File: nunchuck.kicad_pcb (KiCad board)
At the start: 2 copper layers, 117.9 x 118.2 mm, 56 parts, among them J2 USB_C_Receptacle_USB2.0_14P, J3 USB_C_Receptacle_USB2.0_14P, SW1 BOOT, SW2 RESET, SW3 BOOT, SW4 RESET, U1 CH552T, U2 CH552T, U3 USBLC6-2SC6, U4 USBLC6-2SC6

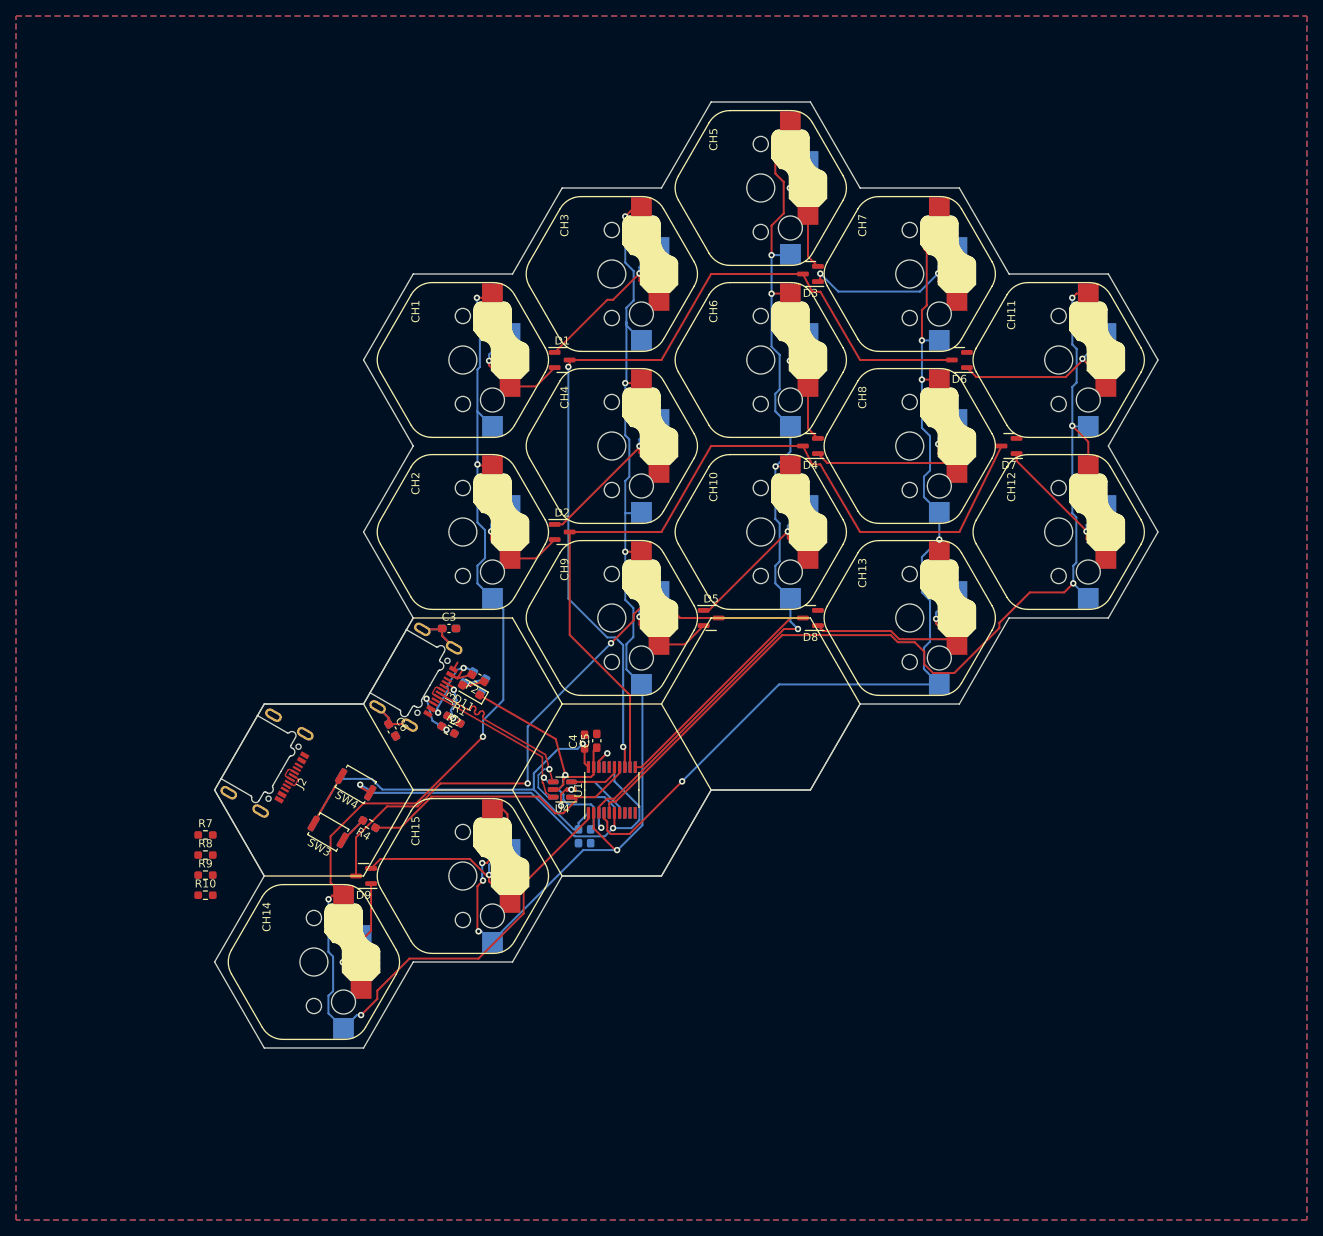
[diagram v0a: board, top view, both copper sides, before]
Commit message: before hexing
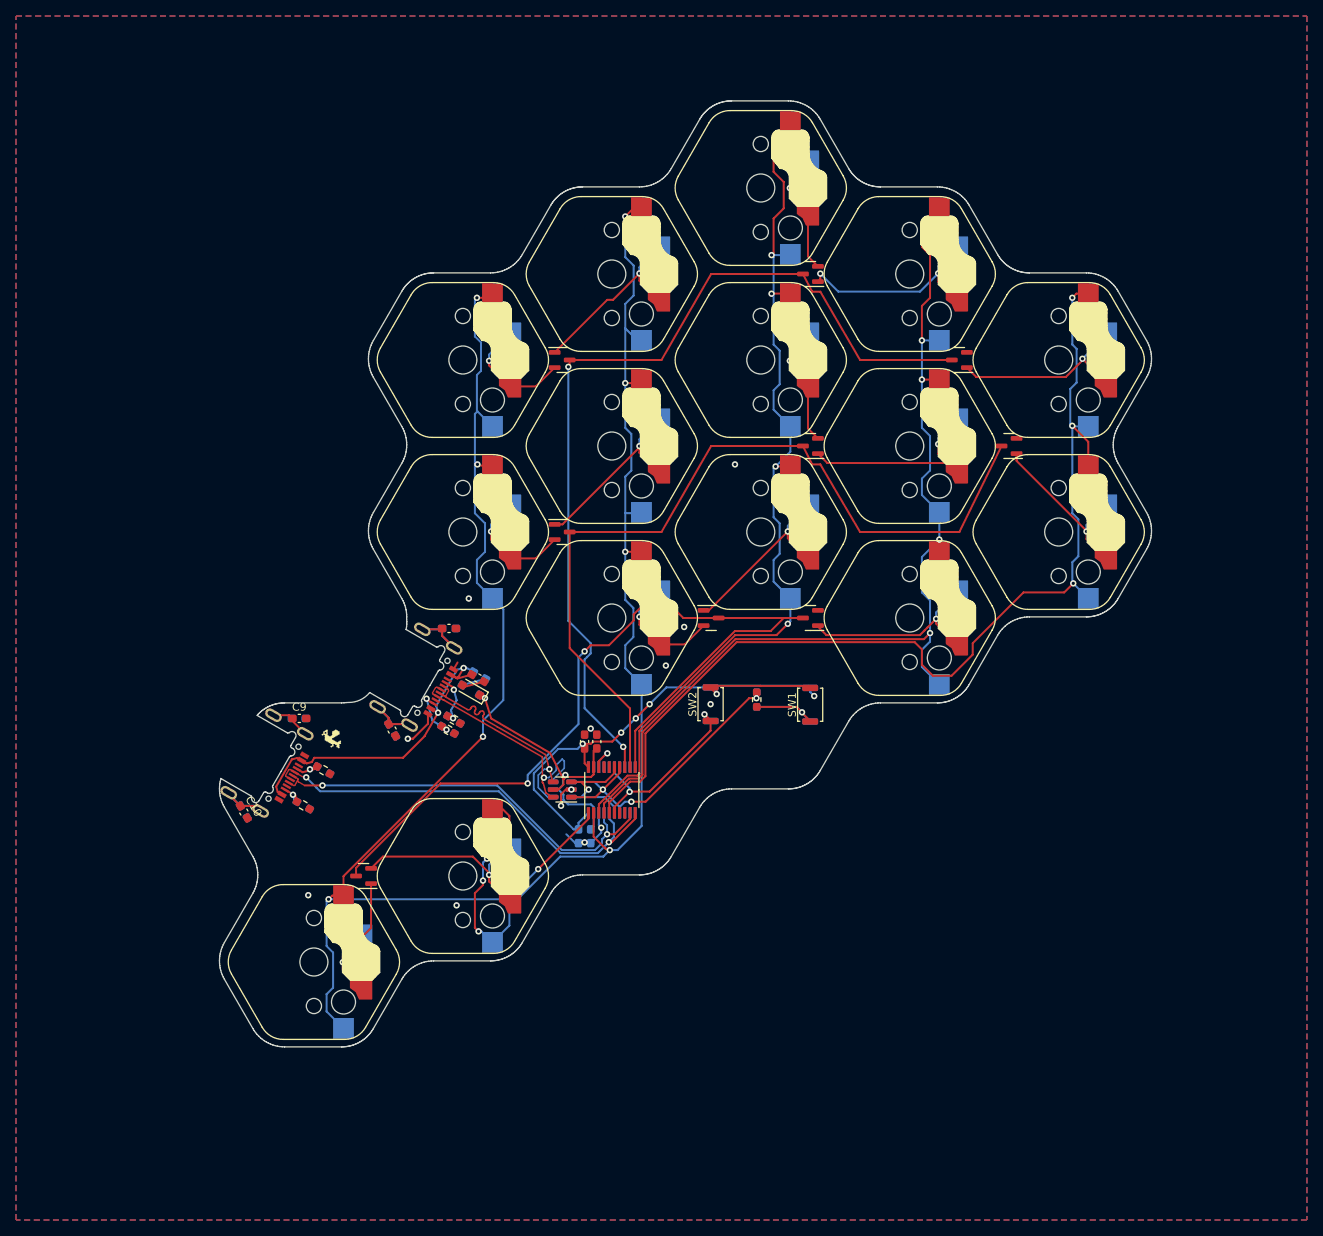
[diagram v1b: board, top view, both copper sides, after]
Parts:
- added C10: 1uF, Capacitor_SMD:C_0603_1608Metric_Pad1.08x0.95mm_HandSolder, F.Cu at (59.5, 110.3)
- added C11: 1uF, Capacitor_SMD:C_0603_1608Metric_Pad1.08x0.95mm_HandSolder, B.Cu at (59.5, 110.2)
- added C12: 1uF, Capacitor_SMD:C_0603_1608Metric_Pad1.08x0.95mm_HandSolder, B.Cu at (66.4, 98.6)
- added C9: 1uF, Capacitor_SMD:C_0603_1608Metric_Pad1.08x0.95mm_HandSolder, F.Cu at (66.4, 98.6)
- R10, R9, SW3, SW4: moved to B.Cu
- SW1, SW2: moved to F.Cu
- moved SW1 62.3 mm to (130.3, 96.8), turned to 90 degrees
- moved SW3 62.3 mm to (130.3, 96.8), turned to 90 degrees
- moved R3 50.9 mm to (123.6, 96.2), turned to -90 degrees
- moved R4 50.9 mm to (123.6, 96.2), turned to -90 degrees
- moved SW2 45.5 mm to (117.9, 96.8), turned to 90 degrees
- moved SW4 45.5 mm to (117.9, 96.8), turned to 90 degrees
- moved R9 19.8 mm to (69.5, 105.0), turned to -30 degrees
- moved R7 16.8 mm to (69.5, 105.0), turned to -30 degrees
- moved R10 16.6 mm to (66.9, 109.4), turned to 150 degrees
- moved R8 13.7 mm to (66.9, 109.4), turned to -30 degrees
- moved D10 0.36 mm to (87.9, 95.0)
- moved C5 0.10 mm to (103.6, 101.4)
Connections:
- J2 pad S1: unconnected-(J2-SHIELD-PadS1) -> Net-(J2-SHIELD)
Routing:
- net TX_L_RX_R: track 2.58 -> 55.9 mm, vias 0 -> 2
- net RX_L_TX_R: track 2.53 -> 53.1 mm, vias 0 -> 2
- net VBUS: track 14.6 -> 41.5 mm
- net RST: track 49.7 -> 24.2 mm
- net Net-(J2-SHIELD): track 0.00 -> 15.2 mm
- net c1: track 161.1 -> 149.4 mm
- net +3.3V: track 61.6 -> 71.4 mm, vias 1 -> 6
- net GND: track 8.67 -> 17.7 mm, vias 4 -> 14
- net BOOT: track 7.13 -> 15.3 mm, vias 0 -> 1
- net r3: track 105.5 -> 112.0 mm
- net PORT+: track 24.6 -> 30.8 mm
- net UDM: track 13.2 -> 18.3 mm, vias 0 -> 1
- net UDP: track 44.7 -> 40.3 mm, vias 0 -> 3
- net Net-(J2-CC1): track 0.00 -> 3.99 mm, vias 0 -> 1
- net c5: track 125.0 -> 129.0 mm
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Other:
- board size 117.9 x 118.2 mm -> 116.5 x 118.2 mm
